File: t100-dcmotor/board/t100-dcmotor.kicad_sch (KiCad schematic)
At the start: 17 parts, among them J1 T100-IN, J2 T100-OUT, J3 Conn_01x08_Female, U1 ATSAMD11D14A-SS, U2 TB67H451FNG, X1 SWD

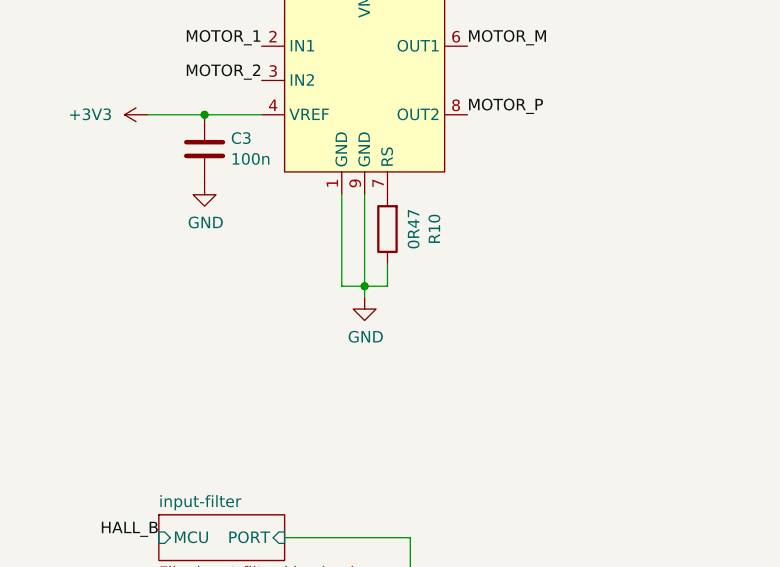
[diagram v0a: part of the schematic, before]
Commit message: WIP
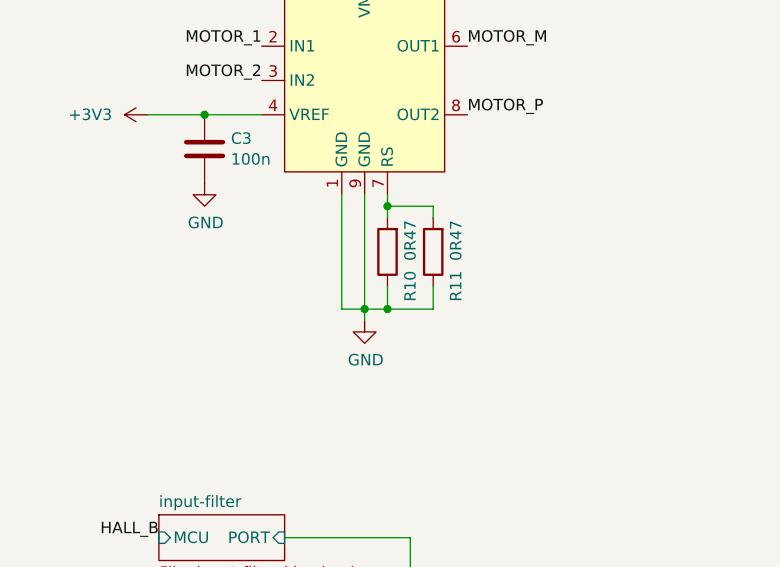
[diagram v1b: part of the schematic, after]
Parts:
- added R11: 0R47, Resistor_SMD:R_0805_2012Metric_Pad1.20x1.40mm_HandSolder, symbol Device:R
- R10: footprint Resistor_SMD:R_1206_3216Metric_Pad1.30x1.75mm_HandSolder -> Resistor_SMD:R_0805_2012Metric_Pad1.20x1.40mm_HandSolder
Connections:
- net GND: now also R11.1
- net at R10.2, U2.7 (RS): now also R11.2
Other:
- moved on the sheet: R10
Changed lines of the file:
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@@
   (junction (at 57.15 72.39) (diameter 0) (color 0 0 0 0)
   )
+  (junction (at 232.41 74.93) (diameter 0) (color 0 0 0 0)
+  )
   (junction (at 50.8 52.07) (diameter 0) (color 0 0 0 0)
   )
@@
   (junction (at 57.15 48.26) (diameter 0) (color 0 0 0 0)
   )
+  (junction (at 232.41 86.36) (diameter 0) (color 0 0 0 0)
+  )
   (junction (at 50.8 72.39) (diameter 0) (color 0 0 0 0)
   )
   (junction (at 63.5 52.07) (diameter 0) (color 0 0 0 0)
   )
-  (junction (at 229.87 83.82) (diameter 0) (color 0 0 0 0)
+  (junction (at 229.87 86.36) (diameter 0) (color 0 0 0 0)
   )
   (no_connect (at 110.49 60.96))
@@
     (stroke (width 0) (type default) (color 0 0 0 0))
   )
+  (wire (pts (xy 237.49 86.36) (xy 237.49 83.82))
+    (stroke (width 0) (type default) (color 0 0 0 0))
+  )
   (wire (pts (xy 149.86 127) (xy 152.4 127))
     (stroke (width 0) (type default) (color 0 0 0 0))
@@
     (stroke (width 0) (type default) (color 0 0 0 0))
   )
-  (wire (pts (xy 232.41 81.28) (xy 232.41 83.82))
+  (wire (pts (xy 232.41 83.82) (xy 232.41 86.36))
     (stroke (width 0) (type default) (color 0 0 0 0))
   )
@@
     (stroke (width 0) (type default) (color 0 0 0 0))
   )
-  (wire (pts (xy 232.41 83.82) (xy 229.87 83.82))
-    (stroke (width 0) (type default) (color 0 0 0 0))
-  )
-  (wire (pts (xy 229.87 73.66) (xy 229.87 83.82))
+  (wire (pts (xy 232.41 86.36) (xy 229.87 86.36))
+    (stroke (width 0) (type default) (color 0 0 0 0))
+  )
+  (wire (pts (xy 229.87 73.66) (xy 229.87 86.36))
+    (stroke (width 0) (type default) (color 0 0 0 0))
+  )
+  (wire (pts (xy 237.49 74.93) (xy 237.49 76.2))
     (stroke (width 0) (type default) (color 0 0 0 0))
   )
@@
     (stroke (width 0) (type default) (color 0 0 0 0))
   )
+  (wire (pts (xy 232.41 74.93) (xy 237.49 74.93))
+    (stroke (width 0) (type default) (color 0 0 0 0))
+  )
   (wire (pts (xy 187.96 129.54) (xy 246.38 129.54))
     (stroke (width 0) (type default) (color 0 0 0 0))
@@
     (stroke (width 0) (type default) (color 0 0 0 0))
   )
+  (wire (pts (xy 232.41 86.36) (xy 237.49 86.36))
+    (stroke (width 0) (type default) (color 0 0 0 0))
+  )
   (wire (pts (xy 50.8 48.26) (xy 57.15 48.26))
     (stroke (width 0) (type default) (color 0 0 0 0))
@@
     (stroke (width 0) (type default) (color 0 0 0 0))
   )
-  (wire (pts (xy 227.33 73.66) (xy 227.33 83.82))
-    (stroke (width 0) (type default) (color 0 0 0 0))
-  )
-  (wire (pts (xy 227.33 83.82) (xy 229.87 83.82))
-    (stroke (width 0) (type default) (color 0 0 0 0))
-  )
-  (wire (pts (xy 229.87 83.82) (xy 229.87 85.09))
+  (wire (pts (xy 227.33 73.66) (xy 227.33 86.36))
+    (stroke (width 0) (type default) (color 0 0 0 0))
+  )
+  (wire (pts (xy 227.33 86.36) (xy 229.87 86.36))
+    (stroke (width 0) (type default) (color 0 0 0 0))
+  )
+  (wire (pts (xy 229.87 86.36) (xy 229.87 87.63))
     (stroke (width 0) (type default) (color 0 0 0 0))
   )
   (wire (pts (xy 233.68 127) (xy 233.68 123.19))
+    (stroke (width 0) (type default) (color 0 0 0 0))
+  )
+  (wire (pts (xy 232.41 76.2) (xy 232.41 74.93))
+    (stroke (width 0) (type default) (color 0 0 0 0))
+  )
+  (wire (pts (xy 232.41 74.93) (xy 232.41 73.66))
     (stroke (width 0) (type default) (color 0 0 0 0))
   )
@@
     (pin "1")
   )
-  (symbol (lib_id "power:GND") (at 229.87 85.09 0) (unit 1)
-    (in_bom yes) (on_board yes)
-    (property "Reference" "#PWR023" (id 0) (at 229.87 91.44 0)
-      (effects (font (size 1.27 1.27)) hide)
-    )
-    (property "Value" "GND" (id 1) (at 229.997 89.4842 0))
-    (property "Footprint" "" (id 2) (at 229.87 85.09 0)
-      (effects (font (size 1.27 1.27)) hide)
-    )
-    (property "Datasheet" "" (id 3) (at 229.87 85.09 0)
+  (symbol (lib_id "power:GND") (at 229.87 87.63 0) (unit 1)
+    (in_bom yes) (on_board yes)
+    (property "Reference" "#PWR023" (id 0) (at 229.87 93.98 0)
+      (effects (font (size 1.27 1.27)) hide)
+    )
+    (property "Value" "GND" (id 1) (at 229.997 92.0242 0))
+    (property "Footprint" "" (id 2) (at 229.87 87.63 0)
+      (effects (font (size 1.27 1.27)) hide)
+    )
+    (property "Datasheet" "" (id 3) (at 229.87 87.63 0)
       (effects (font (size 1.27 1.27)) hide)
     )
@@
     (pin "1")
   )
+  (symbol (lib_id "Device:R") (at 237.49 80.01 180) (unit 1)
+    (in_bom yes) (on_board yes)
+    (property "Reference" "R11" (id 0) (at 240.03 83.82 90))
+    (property "Value" "0R47" (id 1) (at 240.03 78.74 90))
+    (property "Footprint" "Resistor_SMD:R_0805_2012Metric_Pad1.20x1.40mm_HandSolder" (id 2) (at 239.268 80.01 90)
+      (effects (font (size 1.27 1.27)) hide)
+    )
+    (property "Datasheet" "~" (id 3) (at 237.49 80.01 0)
+      (effects (font (size 1.27 1.27)) hide)
+    )
+    (pin "1")
+    (pin "2")
+  )
   (symbol (lib_id "power:GND") (at 212.09 72.39 0) (unit 1)
     (in_bom yes) (on_board yes)
@@
     (pin "1")
   )
-  (symbol (lib_id "Device:R") (at 232.41 77.47 180) (unit 1)
-    (in_bom yes) (on_board yes)
-    (property "Reference" "R10" (id 0) (at 237.6678 77.47 90))
-    (property "Value" "0R47" (id 1) (at 235.3564 77.47 90))
-    (property "Footprint" "Resistor_SMD:R_1206_3216Metric_Pad1.30x1.75mm_HandSolder" (id 2) (at 234.188 77.47 90)
-      (effects (font (size 1.27 1.27)) hide)
-    )
-    (property "Datasheet" "~" (id 3) (at 232.41 77.47 0)
+  (symbol (lib_id "Device:R") (at 232.41 80.01 180) (unit 1)
+    (in_bom yes) (on_board yes)
+    (property "Reference" "R10" (id 0) (at 234.95 83.82 90))
+    (property "Value" "0R47" (id 1) (at 234.95 78.74 90))
+    (property "Footprint" "Resistor_SMD:R_0805_2012Metric_Pad1.20x1.40mm_HandSolder" (id 2) (at 234.188 80.01 90)
+      (effects (font (size 1.27 1.27)) hide)
+    )
+    (property "Datasheet" "~" (id 3) (at 232.41 80.01 0)
       (effects (font (size 1.27 1.27)) hide)
     )
@@
     )
     (path "/9cf70606-6446-435e-8baf-5f19b839292d"
-      (reference "R10") (unit 1) (value "0R47") (footprint "Resistor_SMD:R_1206_3216Metric_Pad1.30x1.75mm_HandSolder")
+      (reference "R10") (unit 1) (value "0R47") (footprint "Resistor_SMD:R_0805_2012Metric_Pad1.20x1.40mm_HandSolder")
+    )
+    (path "/4f7770dd-4b94-4adc-acb1-e53a5fecd595"
+      (reference "R11") (unit 1) (value "0R47") (footprint "Resistor_SMD:R_0805_2012Metric_Pad1.20x1.40mm_HandSolder")
     )
     (path "/00000000-0000-0000-0000-0000606e4326"
